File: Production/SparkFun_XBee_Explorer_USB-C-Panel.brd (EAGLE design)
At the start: 35.6 x 59.7 mm, 109 parts, among them J3 USB Female Type C Connector, J4 QWIIC_RIGHT_ANGLE, U2 AP63203, U5 ESD Diode, U7 FT231XS

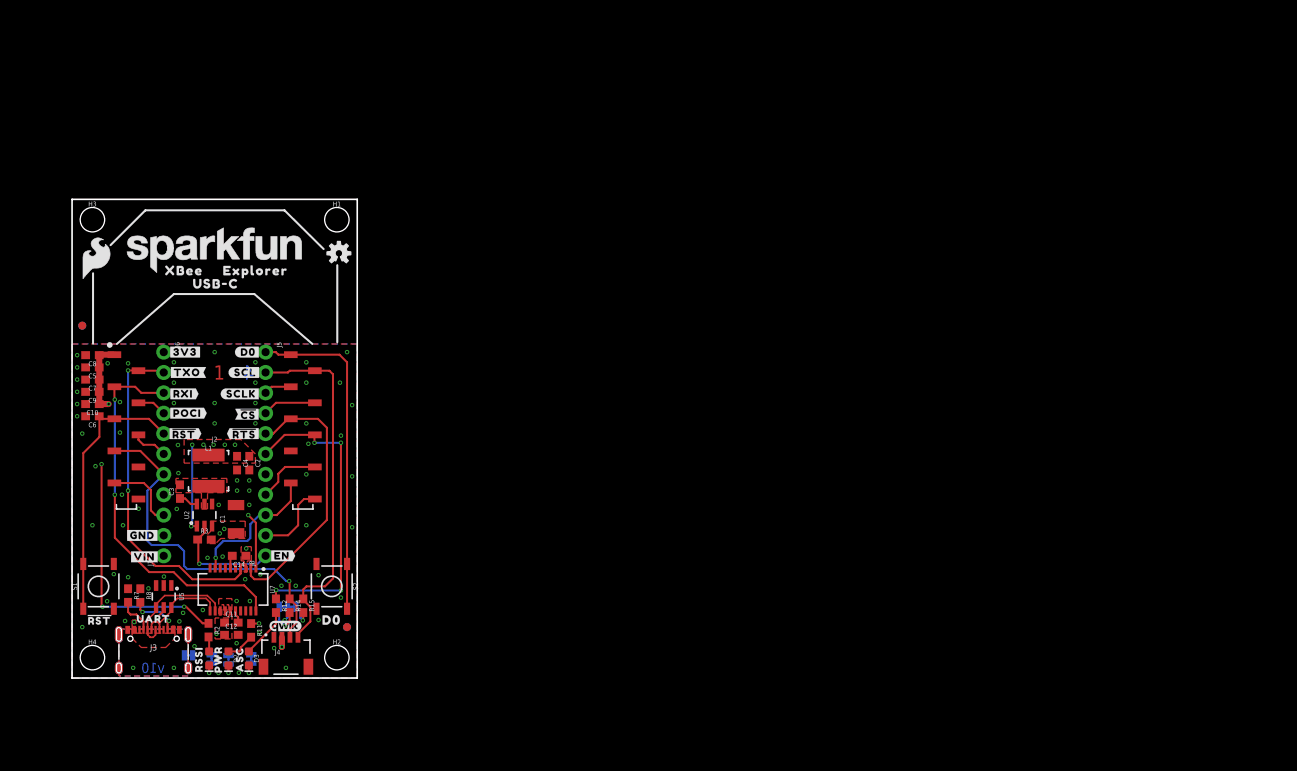
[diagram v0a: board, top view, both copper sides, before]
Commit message: Adds Production Files
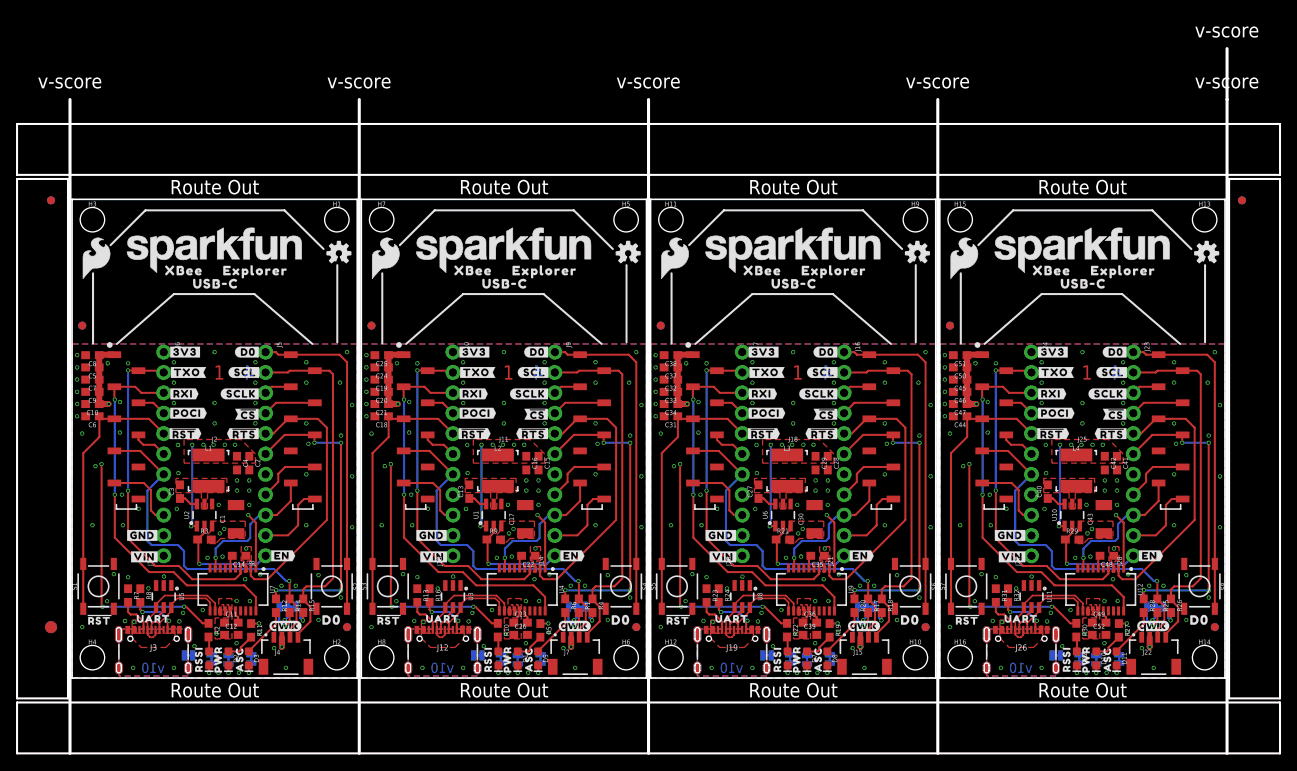
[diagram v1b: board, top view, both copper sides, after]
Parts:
- removed FRAME1: FRAME-LEDGER, SparkFun-Aesthetics:CREATIVE_COMMONS
- added ALED1, ALED2, ALED3, PLED1, PLED2, PLED3, RLED1, RLED2, RLED3, SHLD1, SHLD2, SHLD3: JUMPER-SMT_2_NC_TRACE_SILK, SparkFun-Jumpers:SMT-JUMPER_2_NC_TRACE_SILK
- added C13, C20, C22, C23, C27, C33, C35, C36, C40, C46, C48, C49: 0.1uF, SparkFun-Capacitors:0603
- added C15, C16, C28, C29, C41, C42: 22uF, SparkFun-Capacitors:0603
- added C17, C30, C43: 10uF, SparkFun-Capacitors:1210
- added C18, C19, C31, C32, C44, C45: 10nF, SparkFun-Capacitors:0603
- added C21, C34, C47: 10uF, SparkFun-Capacitors:0603
- added C24, C37, C50: 47pF, SparkFun-Capacitors:0603
- added C25, C38, C51: 10pF, SparkFun-Capacitors:0603
- added C26, C39, C52: 4.7uF, SparkFun-Capacitors:0603
- added D1, D10, D7: Red, SparkFun-LED:LED-0603
- added D11, D5, D8: BLUE, SparkFun-LED:LED-0603
- added D12, D6, D9: Yellow, SparkFun-LED:LED-0603
- added E$1, E$2, E$3, E$4: (no value), SparkFun-Aesthetics:FIDUCIAL-1X2
- added E$5, E$6: (no value), SparkFun-Retired:FIDUCIAL-1.5X3
- added FD10, FD11, FD12, FD13, FD14, FD15, FD16, FD5, FD6, FD7, FD8, FD9: FIDUCIAL1X2, SparkFun-Aesthetics:FIDUCIAL-1X2
- added H10, H11, H12, H13, H14, H15, H16, H5, H6, H7, H8, H9: STAND-OFFTIGHT, SparkFun-Hardware:STAND-OFF-TIGHT
- added I2C_PU1, I2C_PU2, I2C_PU3: JUMPER-SMT_3_2-NC_TRACE_SILK, SparkFun-Jumpers:SMT-JUMPER_3_2-NC_TRACE_SILK
- added J10, J16, J17, J23, J24, J9: (no value), SparkFun-Connectors:1X10_NO_SILK
- added J11, J18, J25: (no value), xbee_smart_modem:XBEE3-SMD
- added J12, J19, J26: USB Female Type C Connector, SparkFun-Connectors:USB-C-16P-4LAYER-ISOLATED
- added J13, J14, J20, J21, J27, J28: (no value), SparkFun-Connectors:1X01_NO_SILK_STAND
- added J15, J22, J7: QWIIC_RIGHT_ANGLE, SparkFun-Connectors:JST04_1MM_RA
- added L2, L3, L4: 3.9UH, SparkFun-Coils:INDUCTOR_3.9UH
- added LOGO10, LOGO7: OSHW-LOGOS, SparkFun-Aesthetics:OSHW-LOGO-S
- added LOGO11, LOGO5, LOGO8: QWIIC_LOGO_4MM, SparkFun-Aesthetics:QWIIC_4MM
- added LOGO12, LOGO6, LOGO9: SFE_LOGO_NAME.2_INCH, SparkFun-Aesthetics:SFE_LOGO_NAME_.2
- added R1, R10, R17, R18, R20, R22, R25, R26, R28, R30, R4, R6: 2.2k, SparkFun-Resistors:0603
- added R13, R16, R23, R24, R31, R32: 5.1k, SparkFun-Resistors:0603
- added R19, R27, R5: 4.7k, SparkFun-Resistors:0603
- added R21, R29, R9: 10k, SparkFun-Resistors:0603
- added S3, S4, S5, S6, S7, S8: (no value), SparkFun-Switches:TACTILE_SWITCH_SMD_5.2MM
- added U$100, U$125, U$154, U$179, U$208, U$71: (no value), topmirror:#GND#0
- added U$101, U$102, U$155, U$156, U$209, U$210: (no value), top:XBEE340
- added U$103, U$157, U$211: (no value), top:ASC32
- added U$104, U$158, U$212: (no value), top:RSSI31
- added U$105, U$159, U$213: (no value), top:PWR29
- added U$106, U$160, U$214: (no value), topmirror:#D1#AD1#SCL#8
- added U$107, U$108, U$161, U$162, U$215, U$216: (no value), top:EXPLORER1344
- added U$109, U$111, U$163, U$165, U$33, U$39: (no value), top:#3V3#1
- added U$110, U$164, U$34: (no value), top:#I2C#33
- added U$112, U$146, U$166, U$200, U$41, U$92: (no value), top:#VIN#4
- added U$113, U$167, U$42: (no value), bot:D03
- added U$114, U$168, U$43: (no value), top:#RST#30
- added U$115, U$169, U$47: (no value), SparkFun-Aesthetics:SFE_LOGO_NAME_.2
- added U$116, U$170, U$50: (no value), SparkFun-Aesthetics:SFE_LOGO_FLAME_.2
- added U$117, U$171, U$53: (no value), topmirror:#D0#AD0#18
- added U$118, U$172, U$55: (no value), topmirror:#D2#AD2#19
- added U$119, U$173, U$56: (no value), topmirror:#D3#AD3#23
- added U$120, U$174, U$57: (no value), topmirror:#D6##RTS##25
- added U$121, U$175, U$62: (no value), topmirror:#D5#ASSOC#25
- added U$122, U$176, U$68: (no value), topmirror:#D9##SLP##28
- added U$123, U$177, U$69: (no value), topmirror:#D7##CTS##26
- added U$124, U$178, U$70: (no value), topmirror:#D4#PICO#25
- added U$126, U$180, U$72: (no value), topmirror:#D8##DTR##27
- added U$127, U$181, U$73: (no value), topmirror:#RSSI#D10#17
- added U$128, U$182, U$74: (no value), topmirror:#SDA#D11#9
- added U$129, U$183, U$75: (no value), topmirror:##RST##15
- added U$130, U$184, U$76: (no value), topmirror:#POCI#D12#24
- added U$131, U$185, U$77: (no value), topmirror:#RXI#D14#15
- added U$132, U$186, U$78: (no value), topmirror:#TXO#D13#13
- added U$133, U$187, U$79: (no value), topmirror:#EN#17
- added U$134, U$188, U$80: (no value), topmirror:#ALED#21
- added U$135, U$189, U$81: (no value), topmirror:#RLED#22
- added U$136, U$190, U$82: (no value), topmirror:#PLED#20
- added U$137, U$191, U$83: (no value), botmirror:#TXO#8
- added U$138, U$192, U$84: (no value), botmirror:#RXI#7
- added U$139, U$193, U$85: (no value), botmirror:#POCI#32
- added U$140, U$194, U$86: (no value), botmirror:##RST##13
- added U$141, U$195, U$87: (no value), botmirror:##RTS##14
- added U$142, U$196, U$88: (no value), botmirror:##CS##26
- added U$143, U$197, U$89: (no value), botmirror:#SCLK#33
- added U$144, U$198, U$90: (no value), botmirror:#SCL#9
- added U$145, U$199, U$91: (no value), botmirror:#D0#3
- added U$147, U$201, U$93: (no value), botmirror:#EN#15
- added U$148, U$202, U$94: (no value), topmirror:#SHLD#36
- added U$149, U$203, U$95: (no value), topmirror:#NC#1
- added U$150, U$204, U$96: (no value), botmirror:#NC#3
- added U$151, U$152, U$205, U$206, U$97, U$98: (no value), topmirror:USB#C1342
- added U$153, U$207, U$99: (no value), topmirror:UART34
- added U1, U10, U6: AP63203, SparkFun-IC-Power:SOT23-6
- added U11, U3, U8: ESD Diode, SparkFun-DiscreteSemi:SOT-23-6
- added U12, U4, U9: FT231XS, SparkFun-IC-Comms:SSOP20_L
- LOGO4: value SPECIAL_INSTRUCTIONS-ORDERING -> OSHW-LOGOS; device SparkFun-Aesthetics:ORDERING_INSTRUCTIONS -> SparkFun-Aesthetics:OSHW-LOGO-S
- moved LOGO4 25.8 mm to (69.3, 53.0)
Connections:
- new net !RESET!1: C18.1, J10.5, J11.5, S3.1, S3.2
- new net !RESET!2: C31.1, J17.5, J18.5, S5.1, S5.2
- new net !RESET!3: C44.1, J24.5, J25.5, S7.1, S7.2
- new net 3.3V1: C15.1, C16.1, C19.1, C20.1, C21.1, C22.1, C23.1, C24.1, C25.1, C26.1, I2C_PU1.2, J10.1, J11.1, J7.2, L2.P$2, R5.1, U1.1, U4.13, U4.14, U4.15, U4.3
- new net 3.3V2: C28.1, C29.1, C32.1, C33.1, C34.1, C35.1, C36.1, C37.1, C38.1, C39.1, I2C_PU2.2, J15.2, J17.1, J18.1, L3.P$2, R19.1, U6.1, U9.13, U9.14, U9.15, U9.3
- new net 3.3V3: C41.1, C42.1, C45.1, C46.1, C47.1, C48.1, C49.1, C50.1, C51.1, C52.1, I2C_PU3.2, J22.2, J24.1, J25.1, L4.P$2, R27.1, U10.1, U12.13, U12.14, U12.15, U12.3
- new net D+1: J12.A6, J12.B6, U3.6, U4.11
- new net D+2: J19.A6, J19.B6, U8.6, U9.11
- new net D+3: J26.A6, J26.B6, U11.6, U12.11
- new net D-1: J12.A7, J12.B7, U3.4, U4.12
- new net D-2: J19.A7, J19.B7, U8.4, U9.12
- new net D-3: J26.A7, J26.B7, U11.4, U12.12
- new net D1: J11.20, J9.1, S4.1, S4.2
- new net D1/SCL1: J11.19, J7.4, J9.2, R4.1
- new net D1/SCL2: J15.4, J16.2, J18.19, R18.1
- new net D1/SCL3: J22.4, J23.2, J25.19, R26.1
- new net D10/RSSI_PWM1: J10.6, J11.6, R10.1
- new net D10/RSSI_PWM2: J17.6, J18.6, R22.1
- new net D10/RSSI_PWM3: J24.6, J25.6, R30.1
- new net D11/SDA1: J10.7, J11.7, J7.3, R1.1
- new net D11/SDA2: J15.3, J17.7, J18.7, R17.1
- new net D11/SDA3: J22.3, J24.7, J25.7, R25.1
- new net D12/SPI_POCI1: J10.4, J11.4
- new net D12/SPI_POCI2: J17.4, J18.4
- new net D12/SPI_POCI3: J24.4, J25.4
- new net D13/TXO1: J10.2, J11.2, U4.4
- new net D13/TXO2: J17.2, J18.2, U9.4
- new net D13/TXO3: J24.2, J25.2, U12.4
- new net D14/RXI1: J10.3, J11.3, U4.20
- new net D14/RXI2: J17.3, J18.3, U9.20
- new net D14/RXI3: J24.3, J25.3, U12.20
- new net D2: J16.1, J18.20, S6.1, S6.2
- new net D2/SPI_CLK1: J11.18, J9.3
- new net D2/SPI_CLK2: J16.3, J18.18
- new net D2/SPI_CLK3: J23.3, J25.18
- new net D3: J23.1, J25.20, S8.1, S8.2
- new net D3/SPI_!CS!1: J11.17, J9.4
- new net D3/SPI_!CS!2: J16.4, J18.17
- new net D3/SPI_!CS!3: J23.4, J25.17
- new net D4/SPI_PICO1: J11.11, J9.10
- new net D4/SPI_PICO2: J16.10, J18.11
- new net D4/SPI_PICO3: J23.10, J25.11
- new net D5/ASSOCIATE1: J11.15, J9.6, R6.1
- new net D5/ASSOCIATE2: J16.6, J18.15, R20.1
- new net D5/ASSOCIATE3: J23.6, J25.15, R28.1
- new net D6/!RTS!1: J11.16, J9.5, U4.2
- new net D6/!RTS!2: J16.5, J18.16, U9.2
- new net D6/!RTS!3: J23.5, J25.16, U12.2
- new net D7/!CTS!1: J11.12, J9.9, U4.9
- new net D7/!CTS!2: J16.9, J18.12, U9.9
- new net D7/!CTS!3: J23.9, J25.12, U12.9
- new net D8/!DTR!1: J10.9, J11.9, U4.1
- new net D8/!DTR!2: J17.9, J18.9, U9.1
- new net D8/!DTR!3: J24.9, J25.9, U12.1
- new net D9/!SLEEP!1: J11.13, J9.8
- new net D9/!SLEEP!2: J16.8, J18.13
- new net D9/!SLEEP!3: J23.8, J25.13
- new net EN1: J14.1, R9.1, U1.2
- new net EN2: J21.1, R21.1, U6.2
- new net EN3: J28.1, R29.1, U10.2
- new net GND1: ALED1.1, C15.2, C16.2, C17.2, C18.2, C19.2, C20.2, C21.2, C22.2, C23.2, C24.2, C25.2, C26.2, J10.10, J11.10, J12.GND, J12.GND2, J7.1, PLED1.1, R13.1, R16.1, RLED1.1, S3.3, S3.4, S4.3, S4.4, SHLD1.1, U1.4, U3.2, U4.16, U4.6
- new net GND2: ALED2.1, C28.2, C29.2, C30.2, C31.2, C32.2, C33.2, C34.2, C35.2, C36.2, C37.2, C38.2, C39.2, J15.1, J17.10, J18.10, J19.GND, J19.GND2, PLED2.1, R23.1, R24.1, RLED2.1, S5.3, S5.4, S6.3, S6.4, SHLD2.1, U6.4, U8.2, U9.16, U9.6
- new net GND3: ALED3.1, C41.2, C42.2, C43.2, C44.2, C45.2, C46.2, C47.2, C48.2, C49.2, C50.2, C51.2, C52.2, J22.1, J24.10, J25.10, J26.GND, J26.GND2, PLED3.1, R31.1, R32.1, RLED3.1, S7.3, S7.4, S8.3, S8.4, SHLD3.1, U10.4, U11.2, U12.16, U12.6
- new net N$10: D1.A, R5.2
- new net N$14: D5.A, R6.2
- new net N$15: ALED1.2, D5.C
- new net N$16: D1.C, PLED1.2
- new net N$17: C13.1, U1.6
- new net N$18: C13.2, L2.P$1, U1.5
- new net N$19: D6.A, R10.2
- new net N$20: D6.C, RLED1.2
- new net N$22: J12.B5, R16.2
- new net N$24: J12.A5, R13.2
- new net N$25: I2C_PU2.3, R17.2
- new net N$26: I2C_PU2.1, R18.2
- new net N$27: D7.A, R19.2
- new net N$28: D8.A, R20.2
- new net N$29: ALED2.2, D8.C
- new net N$30: D7.C, PLED2.2
- new net N$31: C27.1, U6.6
- new net N$32: C27.2, L3.P$1, U6.5
- new net N$33: D9.A, R22.2
- new net N$34: D9.C, RLED2.2
- new net N$35: J19.B5, R24.2
- new net N$36: J19.A5, R23.2
- new net N$37: I2C_PU3.3, R25.2
- new net N$38: I2C_PU3.1, R26.2
- new net N$39: D10.A, R27.2
- new net N$4: I2C_PU1.3, R1.2
- new net N$40: D11.A, R28.2
- new net N$41: ALED3.2, D11.C
- new net N$42: D10.C, PLED3.2
- new net N$43: C40.1, U10.6
- new net N$44: C40.2, L4.P$1, U10.5
- new net N$45: D12.A, R30.2
- new net N$46: D12.C, RLED3.2
- new net N$47: J26.B5, R32.2
- new net N$48: J26.A5, R31.2
- new net N$9: I2C_PU1.1, R4.2
- new net SHLD1: J12.SHLD1, J12.SHLD2, J12.SHLD3, J12.SHLD4, J12.SHLD5, J12.SHLD6, J12.SHLD7, J12.SHLD8, SHLD1.2
- new net SHLD2: J19.SHLD1, J19.SHLD2, J19.SHLD3, J19.SHLD4, J19.SHLD5, J19.SHLD6, J19.SHLD7, J19.SHLD8, SHLD2.2
- new net SHLD3: J26.SHLD1, J26.SHLD2, J26.SHLD3, J26.SHLD4, J26.SHLD5, J26.SHLD6, J26.SHLD7, J26.SHLD8, SHLD3.2
- new net VIN1: C17.1, J12.VBUS1, J12.VBUS2, J13.1, R9.2, U1.3, U3.5
- new net VIN2: C30.1, J19.VBUS1, J19.VBUS2, J20.1, R21.2, U6.3, U8.5
- new net VIN3: C43.1, J26.VBUS1, J26.VBUS2, J27.1, R29.2, U10.3, U11.5
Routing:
- net D14/RXI3: track 0.00 -> 47.7 mm, vias 0 -> 2
- net D14/RXI2: track 0.00 -> 47.7 mm, vias 0 -> 2
- net D14/RXI1: track 0.00 -> 47.7 mm, vias 0 -> 2
- net D1/SCL3: track 0.00 -> 45.4 mm
- net D1/SCL1: track 0.00 -> 45.4 mm
- net D1/SCL2: track 0.00 -> 45.4 mm
- net D11/SDA2: track 0.00 -> 45.1 mm, vias 0 -> 1
- net D11/SDA1: track 0.00 -> 45.1 mm, vias 0 -> 1
- net D11/SDA3: track 0.00 -> 45.1 mm, vias 0 -> 1
- net D10/RSSI_PWM2: track 0.00 -> 44.8 mm, vias 0 -> 3
- net D10/RSSI_PWM3: track 0.00 -> 44.8 mm, vias 0 -> 3
- net D10/RSSI_PWM1: track 0.00 -> 44.8 mm, vias 0 -> 3
- net D13/TXO3: track 0.00 -> 42.6 mm, vias 0 -> 2
- net D13/TXO2: track 0.00 -> 42.6 mm, vias 0 -> 2
- net D13/TXO1: track 0.00 -> 42.6 mm, vias 0 -> 2
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- added copper zone on layer 1, net 3.3V1
- added copper zone on layer 15, net 3.3V1
- added copper zone on layer 1, net 3.3V2
- added copper zone on layer 15, net 3.3V2
- added copper zone on layer 1, net 3.3V3
- added copper zone on layer 15, net 3.3V3
- added copper zone on layer 1, net GND1
- added copper zone on layer 16, net GND1
- added copper zone on layer 2, net GND1
- added copper zone on layer 1, net GND2
- added copper zone on layer 16, net GND2
- added copper zone on layer 2, net GND2
- added copper zone on layer 1, net GND3
- added copper zone on layer 16, net GND3
- added copper zone on layer 2, net GND3
- added copper zone on layer 1, net N$18
- added copper zone on layer 1, net N$32
- added copper zone on layer 1, net N$44
- added copper zone on layer 1, net SHLD1
- added copper zone on layer 15, net SHLD1
- added copper zone on layer 16, net SHLD1
- added copper zone on layer 2, net SHLD1
- added copper zone on layer 1, net SHLD2
- added copper zone on layer 15, net SHLD2
- added copper zone on layer 16, net SHLD2
- added copper zone on layer 2, net SHLD2
- added copper zone on layer 1, net SHLD3
- added copper zone on layer 15, net SHLD3
- added copper zone on layer 16, net SHLD3
- added copper zone on layer 2, net SHLD3
- added copper zone on layer 1, net VIN1
- added copper zone on layer 1, net VIN2
- added copper zone on layer 1, net VIN3
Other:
- board size 35.6 x 59.7 mm -> 157.5 x 87.9 mm
- board text added: "Route Out"
- board text added: "v-score"
- board text removed: "1.6mm Thickness"
- board text removed: "Elias Santistevan"
- board text removed: "Four Layer Board"
- board text removed: "Lead Free HASL"
- board text removed: "Units in Inches"
